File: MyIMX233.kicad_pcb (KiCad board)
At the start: 2 copper layers, 74.1 x 92 mm, 69 parts, among them IC1 iMX233, IC2 DDR_SDRAM_MT46_x16, J1 USB_A, J2 Micro_SD_Card, P1 P4v2, P2 1v2, P3 VDDA1v8, P4 2v5, P5 3v3, SW1 SWITCH_PUSHBUTTON, Y1 24Mhz

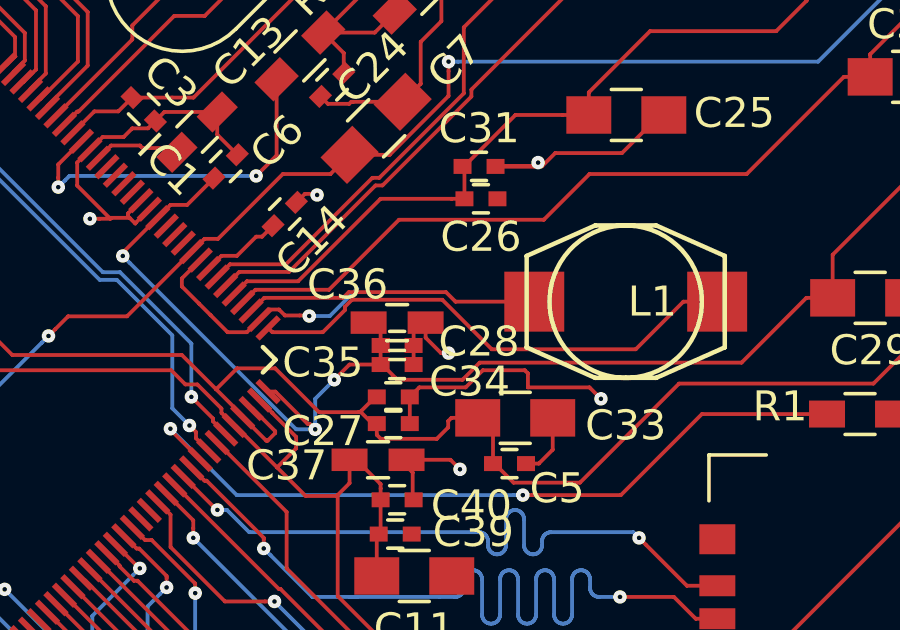
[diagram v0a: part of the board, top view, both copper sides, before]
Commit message: 2nd version
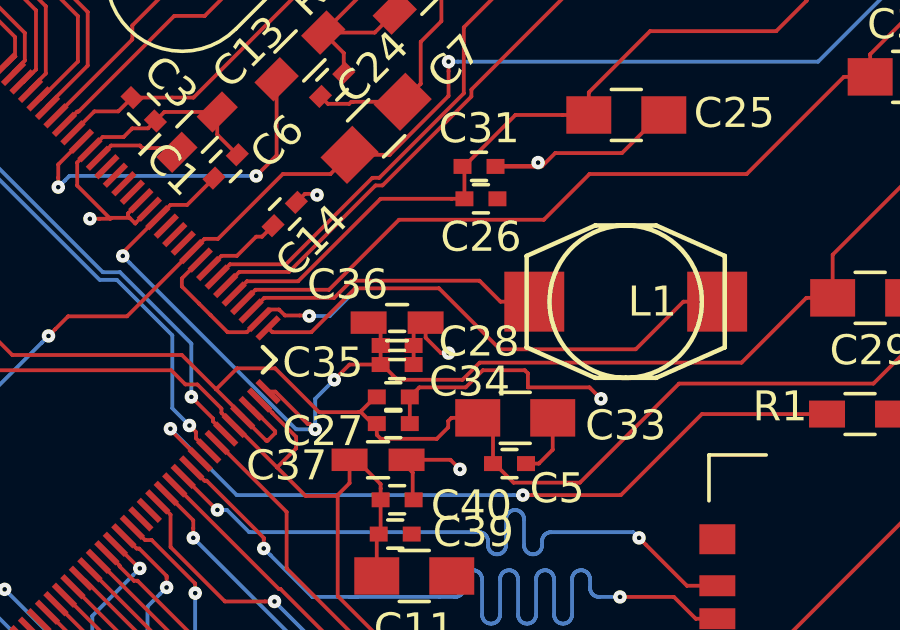
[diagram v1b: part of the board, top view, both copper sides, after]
